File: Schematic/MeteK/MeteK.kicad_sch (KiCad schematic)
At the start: 28 parts, among them J1 Screw_Terminal_01x05, J2 Screw_Terminal_01x02, J3 Conn_01x04_Female, Q1 IRG4PF50W, U1 Pico, U2 LM7805_TO220, U3 HCPL-3120, U4 LM358

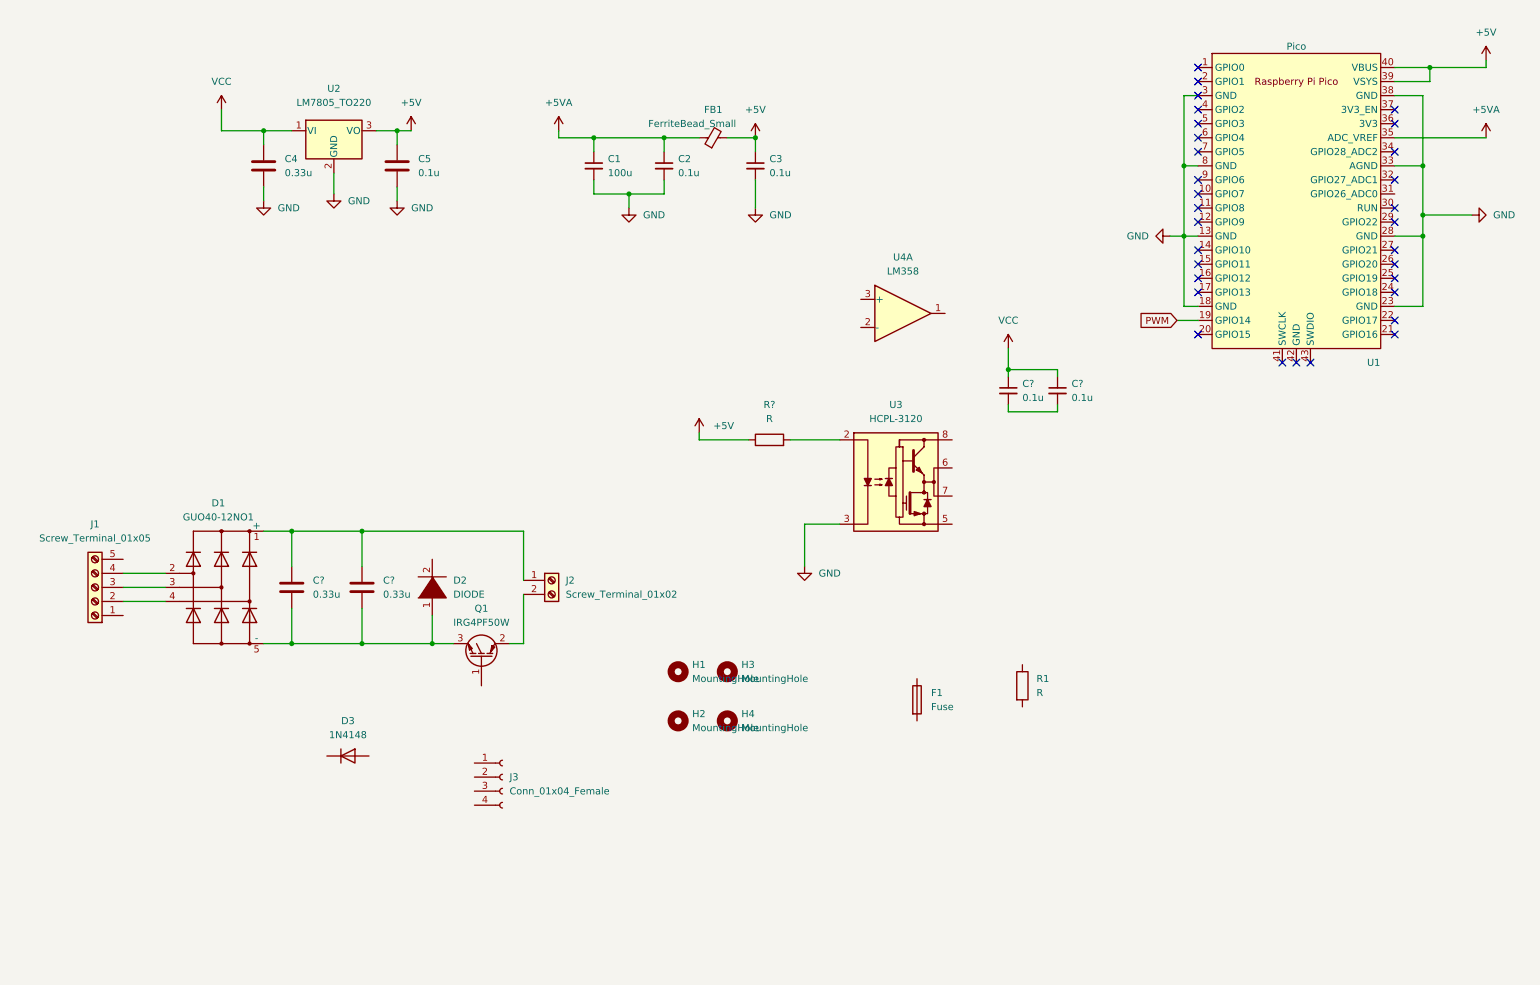
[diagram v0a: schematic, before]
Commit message: further tests on schematic and pcb layout.
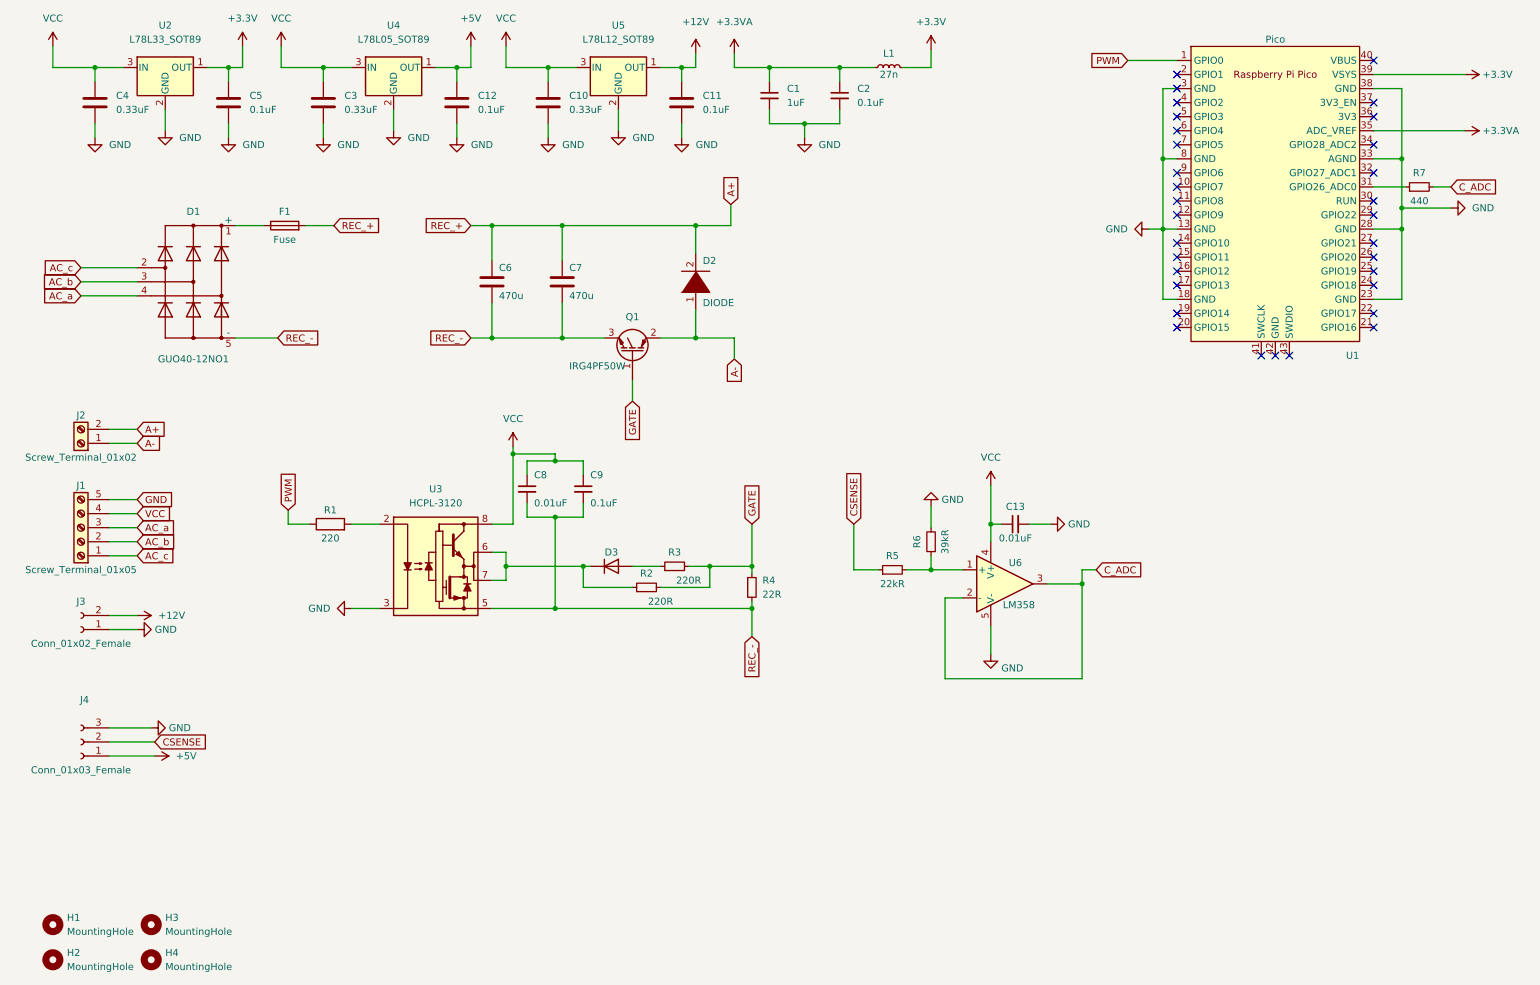
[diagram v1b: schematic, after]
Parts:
- removed C3: 0.1u, Capacitor_THT:C_Disc_D4.3mm_W1.9mm_P5.00mm, symbol Device:C_Small
- removed C? (x2): 0.1u, Capacitor_THT:C_Disc_D14.5mm_W5.0mm_P10.00mm, symbol Device:C_Small
- removed FB1: FerriteBead_Small, Inductor_SMD:L_2512_6332Metric, symbol Device:FerriteBead_Small
- removed J3: Conn_01x04_Female, Connector:FanPinHeader_1x04_P2.54mm_Vertical, symbol Connector:Conn_01x04_Female
- removed R1: R, Resistor_THT:R_Axial_DIN0516_L15.5mm_D5.0mm_P7.62mm_Vertical, symbol Device:R
- removed U2: LM7805_TO220, Package_TO_SOT_THT:TO-220-3_Horizontal_TabDown, symbol Regulator_Linear:LM7805_TO220
- removed U4: LM358, Package_DIP:DIP-8-16_W7.62mm, symbol Amplifier_Operational:LM358
- added C10, C3: 0.33uF, Capacitor_SMD:C_1206_3216Metric, symbol Device:C
- added C11, C12: 0.1uF, Capacitor_SMD:C_1206_3216Metric, symbol Device:C
- added C13, C8: 0.01uF, Capacitor_SMD:C_1206_3216Metric, symbol Device:C_Small
- added C9: 0.1uF, Capacitor_SMD:C_1206_3216Metric, symbol Device:C_Small
- added J3: Conn_01x02_Female, Connector_PinHeader_2.54mm:PinHeader_1x02_P2.54mm_Vertical, symbol Connector:Conn_01x02_Female
- added J4: Conn_01x03_Female, Connector_PinHeader_2.54mm:PinHeader_1x03_P2.54mm_Vertical, symbol Connector:Conn_01x03_Female
- added L1: 27n, Inductor_SMD:L_1206_3216Metric, symbol Device:L_Small
- added R2, R3: 220R, Resistor_SMD:R_0805_2012Metric, symbol Device:R_Small
- added R4: 22R, Resistor_SMD:R_0805_2012Metric, symbol Device:R_Small
- added R5: 22kR, Resistor_SMD:R_0805_2012Metric, symbol Device:R_Small
- added R6: 39kR, Resistor_SMD:R_0805_2012Metric, symbol Device:R_Small
- added R7: 440, Resistor_SMD:R_0805_2012Metric, symbol Device:R_Small
- added U2: L78L33_SOT89, Package_TO_SOT_SMD:SOT-89-3, symbol Regulator_Linear:L78L33_SOT89
- added U4: L78L05_SOT89, Package_TO_SOT_SMD:SOT-89-3, symbol Regulator_Linear:L78L05_SOT89
- added U5: L78L12_SOT89, Package_TO_SOT_SMD:SOT-89-3, symbol Regulator_Linear:L78L12_SOT89
- added U6: LM358, Package_DIP:DIP-8_W7.62mm, symbol pspice:OPAMP
- C1: value 100u -> 1uF; footprint Capacitor_THT:C_Disc_D16.0mm_W5.0mm_P10.00mm -> Capacitor_SMD:C_1206_3216Metric
- C2: value 0.1u -> 0.1uF; footprint Capacitor_THT:C_Disc_D14.5mm_W5.0mm_P10.00mm -> Capacitor_SMD:C_1206_3216Metric
- C4: value 0.33u -> 0.33uF; footprint Capacitor_THT:C_Disc_D3.4mm_W2.1mm_P2.50mm -> Capacitor_SMD:C_1206_3216Metric
- C5: value 0.1u -> 0.1uF; footprint Capacitor_THT:C_Disc_D5.0mm_W2.5mm_P2.50mm -> Capacitor_SMD:C_1206_3216Metric
- C6, C7: renamed from C?; value 0.33u -> 470u; footprint Capacitor_THT:C_Disc_D3.4mm_W2.1mm_P2.50mm -> Capacitor_THT:CP_Radial_D35.0mm_P10.00mm_SnapIn
- D2: footprint Package_TO_SOT_THT:TO-220-2_Horizontal_TabUp -> Package_TO_SOT_THT:TO-220-2_Vertical
- D3: footprint Diode_THT:D_DO-35_SOD27_P7.62mm_Horizontal -> Diode_SMD:D_SMB
- F1: footprint Fuse:Fuse_Bourns_MF-RG1100 -> Fuse:Fuseholder_Clip-5x20mm_Bel_FC-203-22_Lateral_P17.80x5.00mm_D1.17mm_Horizontal
- H1, H2, H3, H4: footprint MountingHole:MountingHole_3.2mm_M3 -> MountingHole:MountingHole_3.2mm_M3_Pad
- R1: renamed from R?; value R -> 220; footprint Resistor_THT:R_Axial_DIN0516_L15.5mm_D5.0mm_P7.62mm_Vertical -> Resistor_SMD:R_0603_1608Metric
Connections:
- net +5V: now also C12.1, J4.1 (Pin_1), U4.1 (OUT); no longer C5.1, R1.1, U1.39 (VSYS), U1.40 (VBUS)
- net GND: now also J1.5 (Pin_5), C10.2, C11.2, C12.2, C13.2, C3.2, J3.1 (Pin_1), J4.3 (Pin_3), R6.2, U2.2 (GND), U4.2 (GND), U5.2 (GND), U6.5 (V-)
- net PWM: now also R1.1, U1.1 (GPIO0); no longer U1.19 (GPIO14)
- net VCC: now also J1.4 (Pin_4), U3.8 (VCC), C10.1, C13.1, C3.1, C8.1, C9.1, U2.3 (IN), U4.3 (IN), U5.3 (IN), U6.4 (V+)
- net A+: now reaches C6.1, C7.1
- net A+: now also D2.2 (A), F1.2, J2.2 (Pin_2); no longer D1.1 (+), J2.1 (Pin_1)
- net REC_-: now reaches C6.2, C7.2, D1.5 (-), Q1.3 (E)
- net REC_-: now also U3.5 (VEE), C8.2, C9.2, R4.2; no longer D2.1 (K)
- net A-: now reaches Q1.2 (C)
- net A-: now also D2.1 (K), J2.1 (Pin_1); no longer J2.2 (Pin_2)
- net at U1.31 (GPIO26_ADC0): now also R7.1
- net GATE: now reaches Q1.1 (G)
- net GATE: now also R2.2, R3.2, R4.1
- net AC_c: now reaches J1.1 (Pin_1)
- net AC_c: now also D1.2
- net AC_a: now reaches D1.4
- net AC_a: now also J1.3 (Pin_3); no longer J1.2 (Pin_2)
- net AC_b: now reaches D1.3
- net AC_b: now also J1.2 (Pin_2); no longer J1.3 (Pin_3)
- net at D3.1 (K): now also U3.6 (VO), U3.7 (VO), R2.1
- net at D3.2 (A): now also R3.1
- net at F1.1: now also D1.1 (+)
- net +5VA renamed +3.3VA
- net +3.3VA: now also L1.1
- new net: R5.2, R6.1, U6.1 (+)
- new net +12V: C11.1, J3.2 (Pin_2), U5.1 (OUT)
- new net +3.3V: C5.1, L1.2, U1.39 (VSYS), U2.1 (OUT)
- new net CSENSE: J4.2 (Pin_2), R5.1
- new net C_ADC: R7.2, U6.2 (-), U6.3
- no-connect marks 31 -> 32
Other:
- moved on the sheet: C1, C2, C4, C5, C6, C7, D1, D2, D3, F1, H1, H2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
